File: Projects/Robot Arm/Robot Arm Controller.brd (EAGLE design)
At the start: 160 x 80 mm, 71 parts, among them IC1 U_FTDICHIP_FT232RL, J1 ICSP HEADER, J2 SERVO PWR, J3 STEPPER, J4 J_MOLEX_502386, P1 P_USB_MINIUX60A-MB-5ST, P2 +12V INPUT, Q1 FDV303N, U1 UA78M05CDCY, U2 TPS71550DCKR, U3 U_ATMEGA328P-AU, U4 U_5VSWITCHER_LM2576SX-5.0, U5 A4988ALT1, U6 U_OPAMP_MCP6001T-E/OT, Y1 CSTCE16M0V13

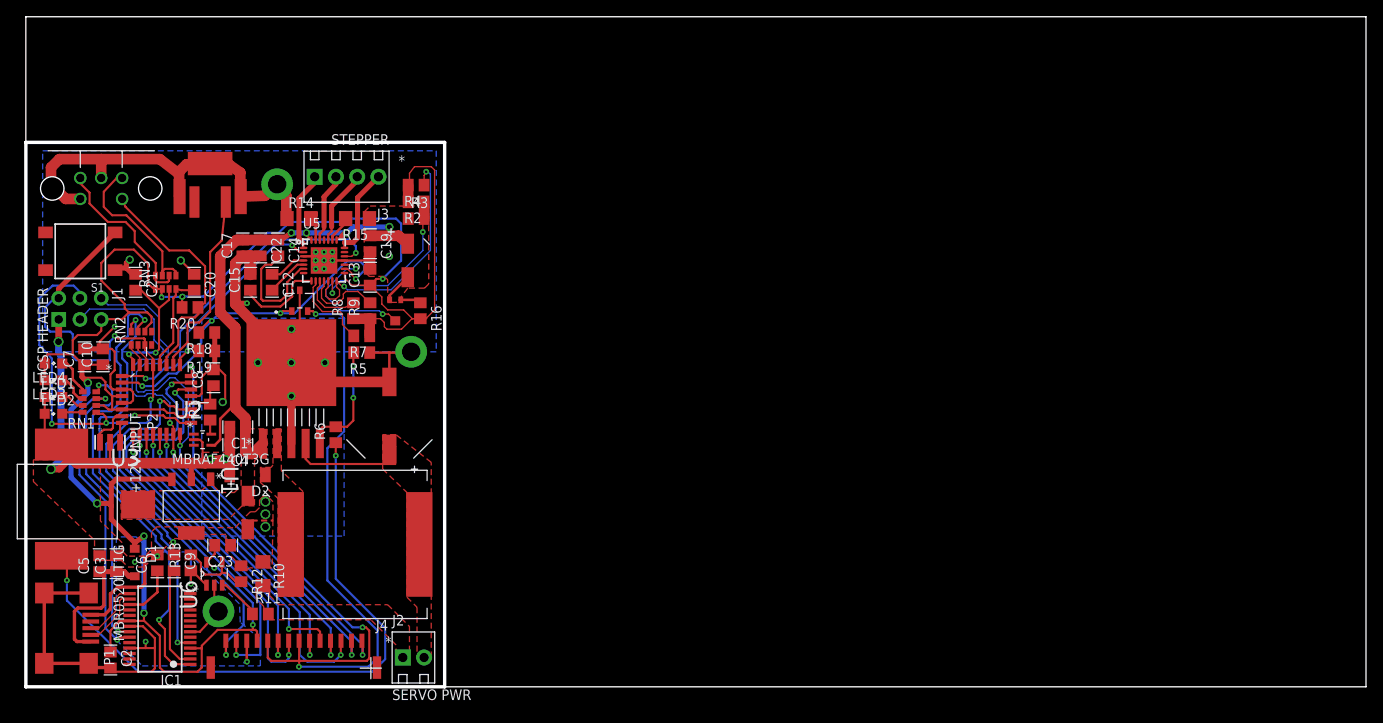
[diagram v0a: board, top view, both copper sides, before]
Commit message: Entire board up for review
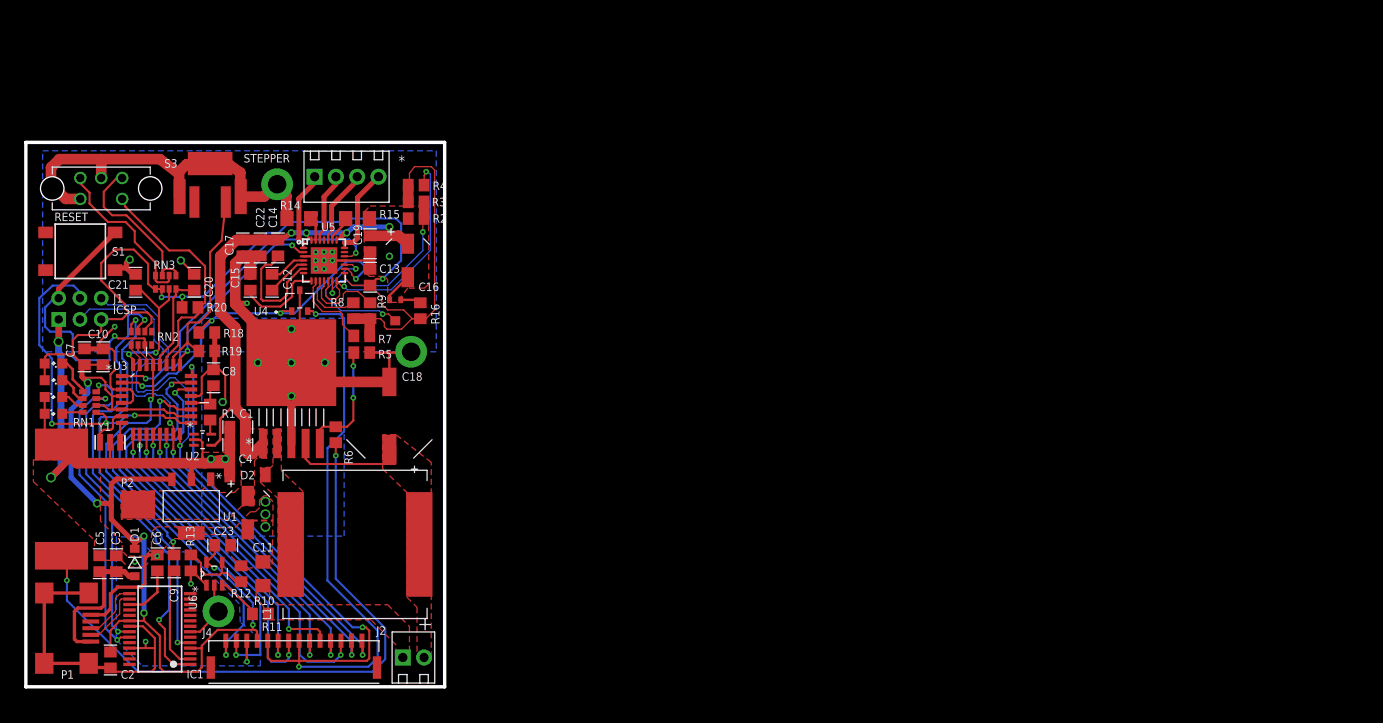
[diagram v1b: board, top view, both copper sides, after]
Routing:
- net GND: track 294.0 -> 295.4 mm
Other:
- board size 160 x 80 mm -> 50 x 65 mm
- board text added: "ICSP"
- board text added: "RESET"
- board text added: "STEPPER"
